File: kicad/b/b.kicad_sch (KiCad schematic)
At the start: 8 parts, among them J1 Conn_01x01_Socket, J2 Conn_01x01_Socket, J3 Conn_01x01_Socket, J4 Conn_01x01_Socket, J5 Conn_01x01_Socket, J6 Conn_01x01_Socket, U1 ABX00012

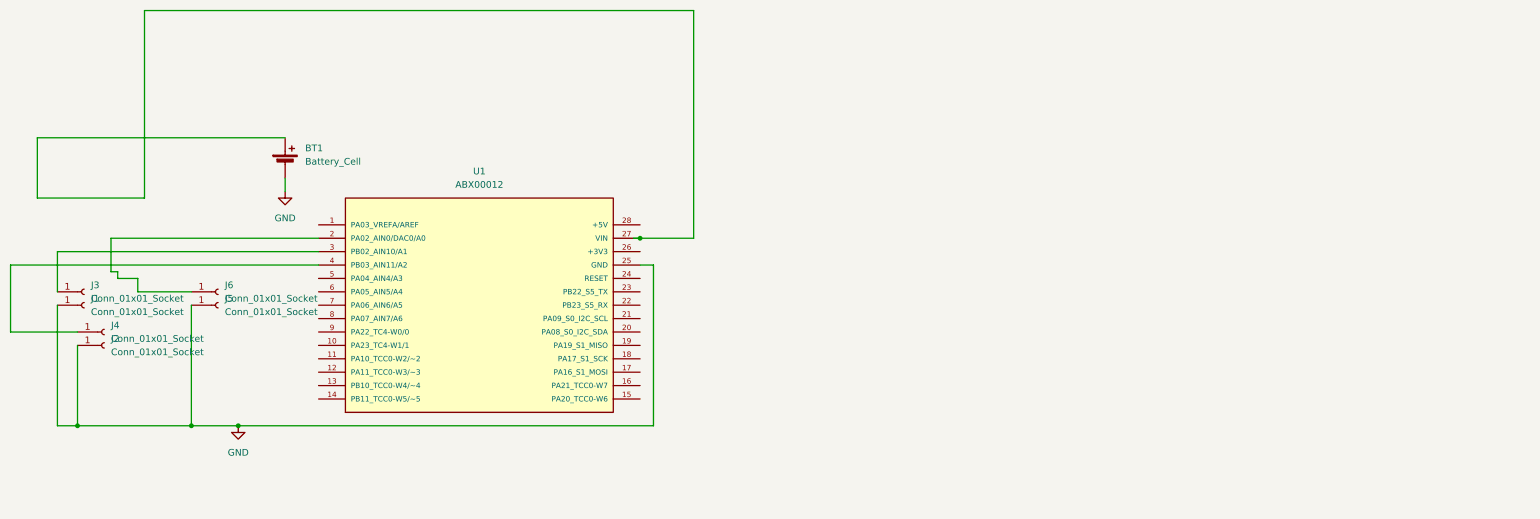
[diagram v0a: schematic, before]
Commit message: kicad done
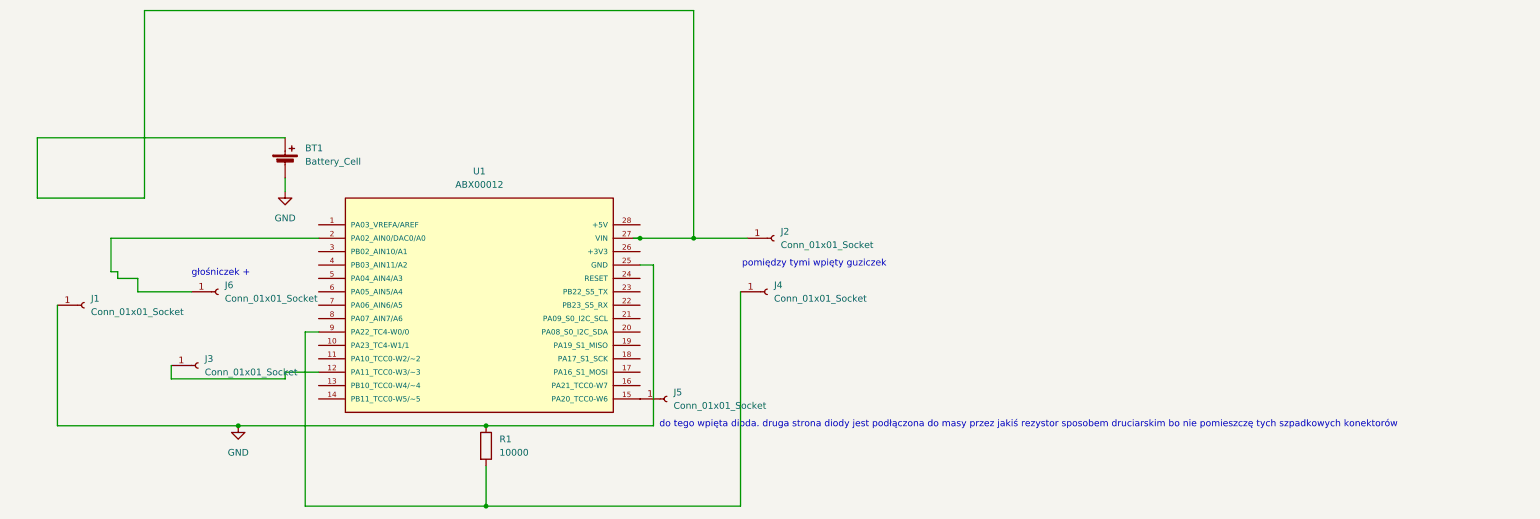
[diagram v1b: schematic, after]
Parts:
- added R1: 10000, Resistor_SMD:R_0201_0603Metric, symbol Device:R
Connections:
- net GND: now also R1.1; no longer J2.1 (Pin_1), J5.1 (Pin_1)
- net at BT1.1 (+), U1.27 (VIN): now also J2.1 (Pin_1)
- net at J3.1 (Pin_1): now also U1.12 (PA11_TCC0-W3/~3); no longer U1.3 (PB02_AIN10/A1)
- net at U1.15 (PA20_TCC0-W6): now also J5.1 (Pin_1)
- net at U1.4 (PB03_AIN11/A2): no longer J4.1 (Pin_1)
- net at U1.9 (PA22_TC4-W0/0): now also J4.1 (Pin_1), R1.2
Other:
- note added: "do tego wpięta dioda. druga strona diody jest podłączona do masy przez jakiś rezystor sposobem druciarskim bo nie pomieszczę tych szpadkowych konektorów"
- note added: "głośniczek +"
- note added: "pomiędzy tymi wpięty guziczek"
